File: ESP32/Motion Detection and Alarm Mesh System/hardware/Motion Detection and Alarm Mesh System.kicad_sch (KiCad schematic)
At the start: 0 parts

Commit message: done with block diagram
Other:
- note added: "(MASTER)"
- note added: "(SLAVE 1)"
- note added: "(SLAVE 2)"
- note added: "(SLAVE 3)"
- note added: "BATTERY"
- note added: "BUZZER"
- note added: "CHARGE AND DISCHAGE MODULE"
- note added: "CHARGER"
- note added: "LED INDICATOR"
- note added: "MICROCONTROLLER WITH WIFI COMPATIBILITY"
- note added: "MOTION SENSOR"
- note added: "VOLTAGE REGULATOR"

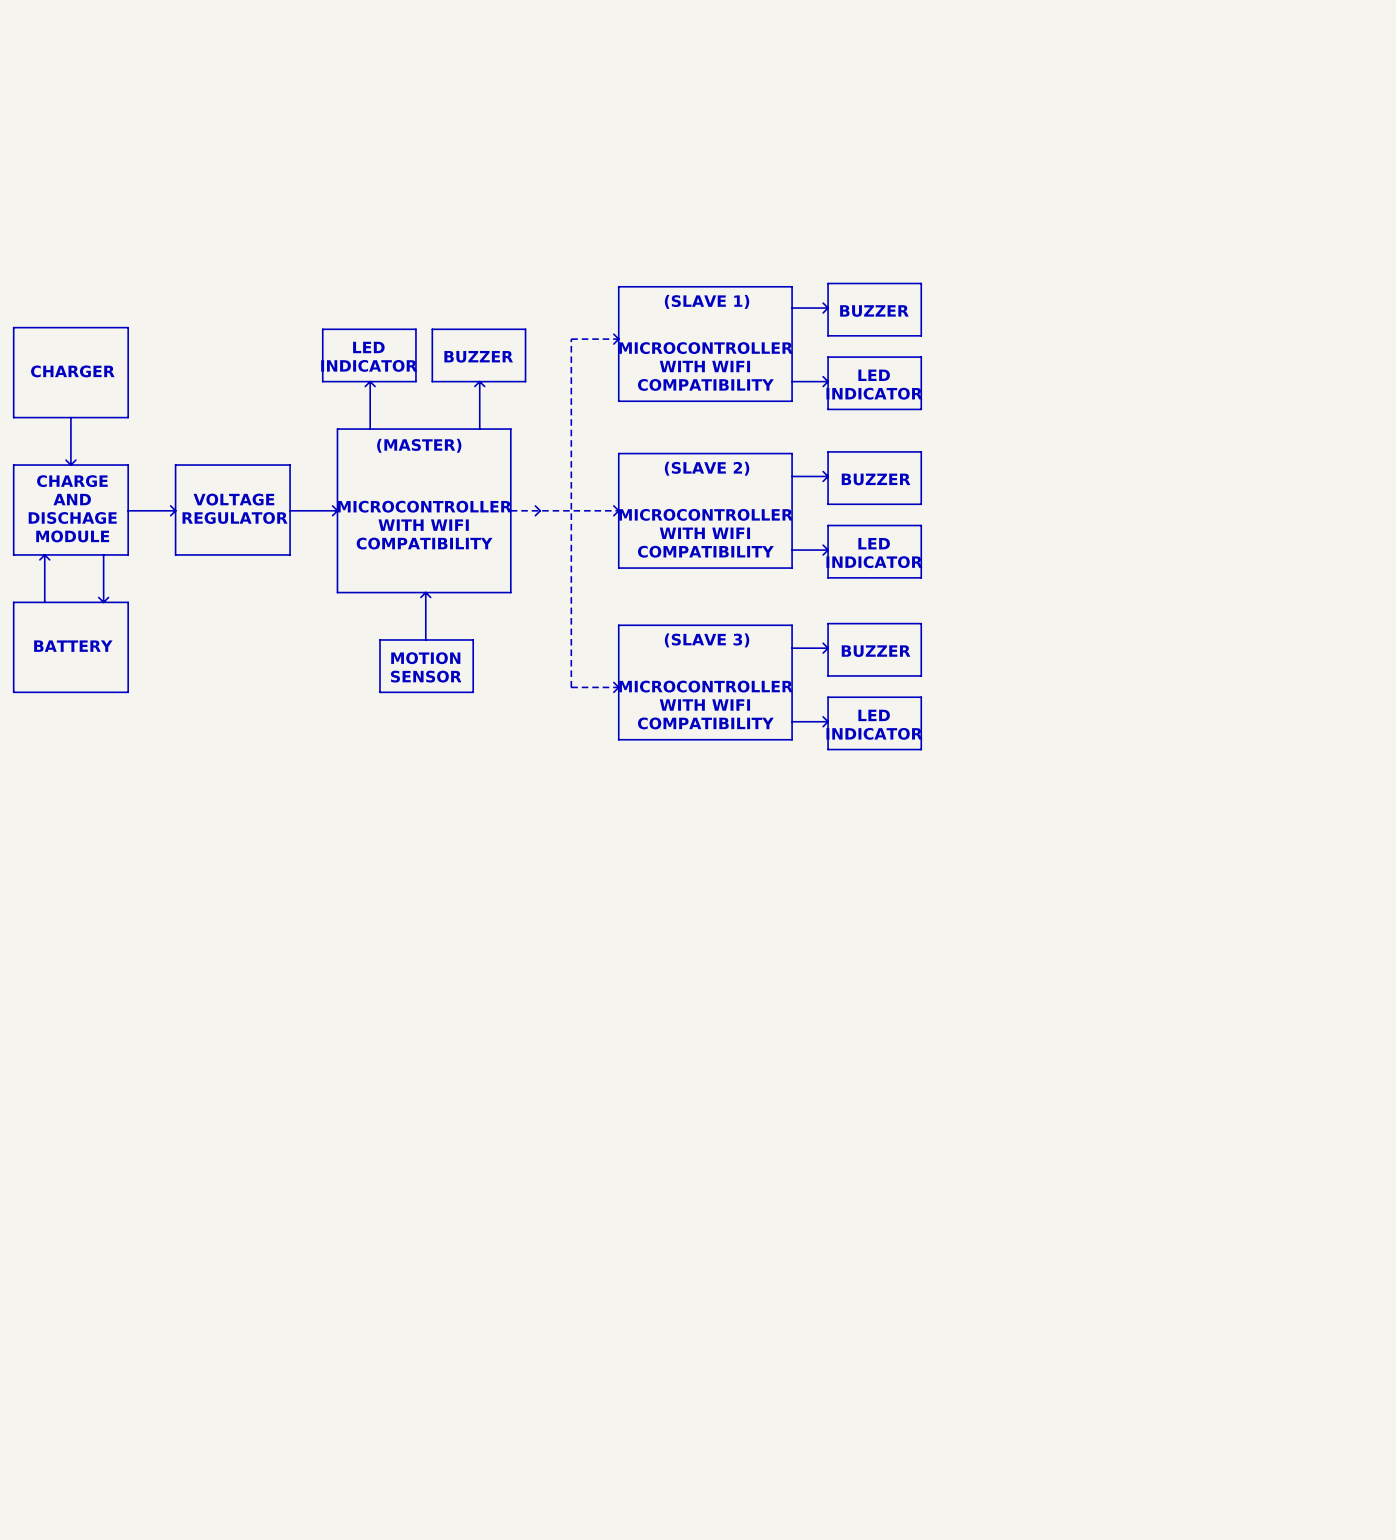
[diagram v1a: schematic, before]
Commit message: Done with Schematic Diagram
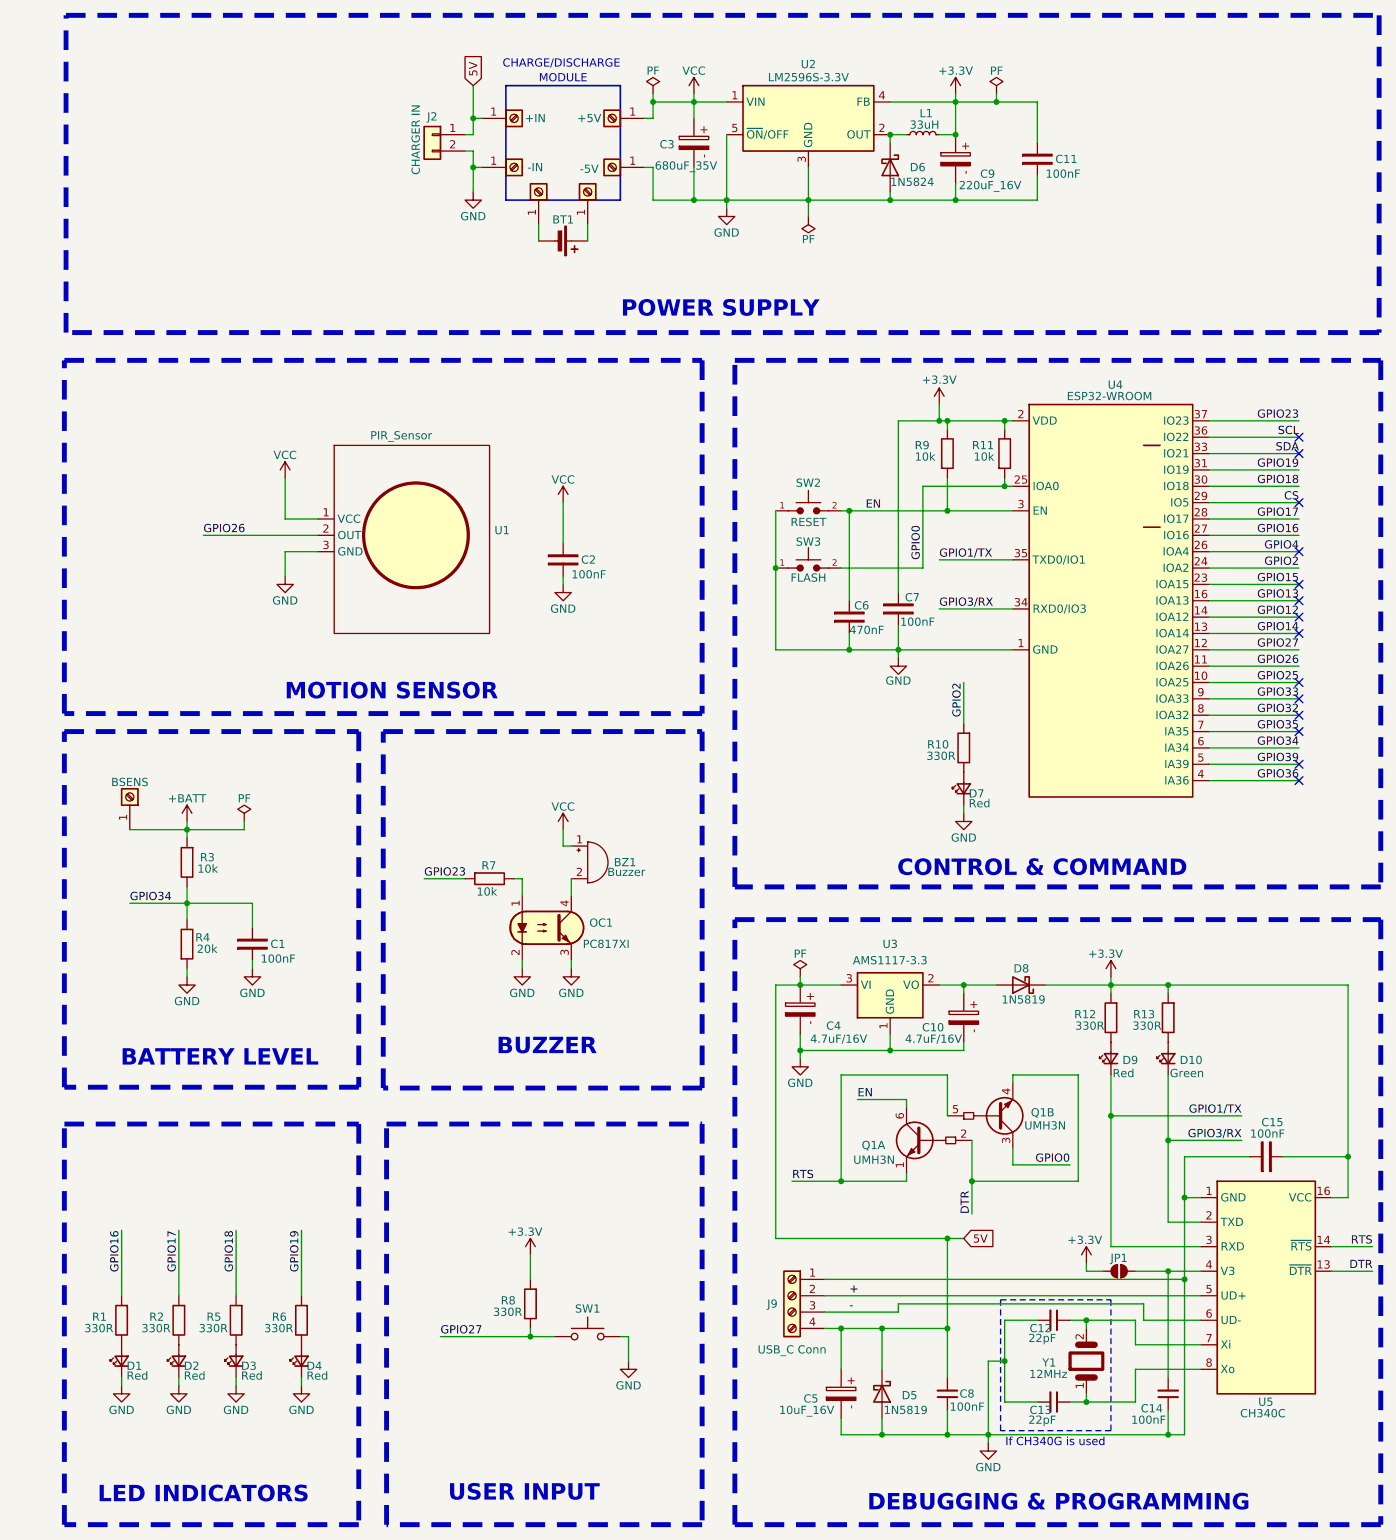
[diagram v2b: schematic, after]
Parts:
- added BT1: Battery_Cell, symbol Device:Battery_Cell
- added BZ1: Buzzer, Buzzer_Beeper:Buzzer_15x7.5RM7.6, symbol Device:Buzzer
- added C1, C11, C15, C2, C7: 100nF, Capacitor_SMD:C_0805_2012Metric_Pad1.18x1.45mm_HandSolder, symbol PCM_SL_Capacitors:104_Ceramic
- added C10, C4: 4.7uF/16V, Capacitor_Tantalum_SMD:CP_EIA-3528-21_Kemet-B_HandSolder, symbol PCM_SL_Capacitors:4.7uF_16V
- added C12, C13: 22pF, Capacitor_SMD:C_0805_2012Metric_Pad1.18x1.45mm_HandSolder, symbol Device:C_Small
- added C14, C8: 100nF, Capacitor_SMD:C_0805_2012Metric_Pad1.18x1.45mm_HandSolder, symbol Device:C_Small
- added C3: 680uF_35V, Capacitor_SMD:CP_Elec_10x12.5, symbol PCM_SL_Capacitors:470uF_35V
- added C5: 10uF_16V, Capacitor_THT:CP_Radial_D5.0mm_P2.00mm, symbol PCM_SL_Capacitors:10uF_16V
- added C6: 470nF, Capacitor_SMD:C_0805_2012Metric_Pad1.18x1.45mm_HandSolder, symbol PCM_SL_Capacitors:104_Ceramic
- added C9: 220uF_16V, Capacitor_SMD:CP_Elec_6.3x7.7, symbol PCM_SL_Capacitors:470uF_35V
- added D1, D2, D3, D4, D7, D9: Red, LED_THT:LED_D3.0mm, symbol SparkFun-LED:LED_Red_0603
- added D10: Green, LED_THT:LED_D3.0mm, symbol SparkFun-LED:LED_Red_0603
- added D5, D8: 1N5819, Diode_SMD:D_SMA, symbol Diode:1N5819
- added D6: 1N5824, Diode_SMD:D_SMA, symbol Diode:1N5822
- added J1: BSENS, Connector_Wire:SolderWire-0.1sqmm_1x01_D0.4mm_OD1mm, symbol Connector:Screw_Terminal_01x01
- added J2: CHARGER IN, symbol Connector_Generic:Conn_01x02
- added J3: +IN, TestPoint:TestPoint_Keystone_5015_Micro_Mini, symbol Connector:Screw_Terminal_01x01
- added J4: -IN, TestPoint:TestPoint_Keystone_5015_Micro_Mini, symbol Connector:Screw_Terminal_01x01
- added J5: -BATT, symbol Connector:Screw_Terminal_01x01
- added J6: +BATT, symbol Connector:Screw_Terminal_01x01
- added J7: +5V, TestPoint:TestPoint_Keystone_5015_Micro_Mini, symbol Connector:Screw_Terminal_01x01
- added J8: -5V, TestPoint:TestPoint_Keystone_5015_Micro_Mini, symbol Connector:Screw_Terminal_01x01
- added J9: USB_C Conn, Connector_PinHeader_2.54mm:PinHeader_1x04_P2.54mm_Vertical, symbol Connector:Screw_Terminal_01x04
- added JP1: ~, Jumper:SolderJumper-2_P1.3mm_Open_Pad1.0x1.5mm, symbol SparkFun-Jumper:SolderJumper_2_Open
- added L1: 33uH, Inductor_SMD:L_12x12mm_H6mm, symbol Device:L_Small
- added OC1: PC817XI, PCM_Package_DIP_AKL:SMDIP-4_W9.53mm, symbol PCM_Optocoupler_AKL:PC817XI
- added Q1: UMH3N, Package_TO_SOT_SMD:SOT-363_SC-70-6, symbol Transistor_BJT:UMH3N
- added R1, R10, R12, R13, R2, R5, R6, R8: 330R, Resistor_SMD:R_0805_2012Metric, symbol PCM_SL_Resistors:1M
- added R11, R3, R7, R9: 10k, Resistor_SMD:R_0805_2012Metric, symbol PCM_SL_Resistors:10k
- added R4: 20k, Resistor_SMD:R_0805_2012Metric, symbol PCM_SL_Resistors:10k
- added SW1: SW_Push, Button_Switch_THT:SW_PUSH_6mm_H13mm, symbol Switch:SW_Push
- added SW2: RESET, Button_Switch_SMD:SW_SPST_CK_KXT3, symbol PCM_SL_Devices:Push_Button
- added SW3: FLASH, Button_Switch_SMD:SW_SPST_CK_KXT3, symbol PCM_SL_Devices:Push_Button
- added U1: PIR_Sensor, PCM_SL_Breakout_Boards:PIR-Sensor, symbol PCM_SL_Breakout_Boards:PIR_Sensor
- added U2: LM2596S-3.3V, Package_TO_SOT_SMD:TO-263-5_TabPin6, symbol Regulator_Switching:LM2596S-3.3
- added U3: AMS1117-3.3, Package_TO_SOT_SMD:SOT-223-3_TabPin2, symbol Regulator_Linear:AMS1117-3.3
- added U4: ESP32-WROOM, RF_Module:ESP32-WROOM-32, symbol SparkFun-RF:ESP32-WROOM
- added U5: CH340C, Package_SO:SOIC-16_3.9x9.9mm_P1.27mm, symbol Interface_USB:CH340C
- added Y1: 12MHz, Crystal:Crystal_HC49-4H_Vertical, symbol PCM_SL_Devices:Crystal_16MHz
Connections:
- new net: C14.2, JP1.1 (A), U5.4 (V3)
- new net: C12.1, U5.7 (Xi), Y1.2
- new net: C13.1, U5.8 (Xo), Y1.1
- new net: OC1.1, R7.2
- new net: D9.2 (A), R12.2
- new net: D3.2 (A), R5.2
- new net: BT1.1 (+), J6.1 (Pin_1)
- new net: C10.1, D8.2 (A), U3.2 (VO)
- new net: D7.2 (A), R10.2
- new net: D2.2 (A), R2.2
- new net: D6.1 (K), L1.1, U2.2 (OUT)
- new net: D1.2 (A), R1.2
- new net: BT1.2 (-), J5.1 (Pin_1)
- new net: BZ1.2 (-), OC1.4
- new net: D4.2 (A), R6.2
- new net: D10.2 (A), R13.2
- new net +: J9.2 (Pin_2), U5.5 (UD+)
- new net +3.3V: C11.2, C15.1, C7.2, C9.1, D8.1 (K), JP1.2 (B), L1.2, R11.2, R12.1, R13.1, R8.1, R9.2, U2.4 (FB), U4.2 (VDD), U5.16 (VCC)
- new net +BATT: J1.1 (Pin_1), R3.1
- new net -: J9.3 (Pin_3), U5.6 (UD-)
- new net 5V: C4.1, C5.1, C8.2, D5.1 (K), J2.1 (Pin_1), J3.1 (Pin_1), J9.4 (Pin_4), U3.3 (VI)
- new net CS: U4.29 (IO5)
- new net DTR: Q1.2 (B1), Q1.4 (E2), U5.13 (~{DTR})
- new net EN: C6.2, Q1.6 (C1), R9.1, SW2.2, U4.3 (EN)
- new net GND: C1.1, C10.2, C11.1, C12.2, C13.2, C14.1, C15.2, C2.1, C3.2, C4.2, C5.2, C6.1, C7.1, C8.1, C9.2, D1.1 (K), D2.1 (K), D3.1 (K), D4.1 (K), D5.2 (A), D6.2 (A), D7.1 (K), J2.2 (Pin_2), J4.1 (Pin_1), J8.1 (Pin_1), J9.1 (Pin_1), OC1.2, OC1.3, R4.1, SW1.2, SW2.1, SW3.1, U1.3 (GND), U2.3 (GND), U2.5 (~{ON}/OFF), U2.6 (GND), U3.1 (GND), U4.1 (GND), U4.15 (GND), U4.38 (GND), U4.39 (GND), U5.1 (GND)
- new net GPIO0: Q1.3 (C2), R11.1, SW3.2, U4.25 (IOA0)
- new net GPIO12: U4.14 (IOA12)
- new net GPIO13: U4.16 (IOA13)
- new net GPIO14: U4.13 (IOA14)
- new net GPIO15: U4.23 (IOA15)
- new net GPIO16: R1.1, U4.27 (IO16)
- new net GPIO17: R2.1, U4.28 (IO17)
- new net GPIO18: R5.1, U4.30 (IO18)
- new net GPIO19: R6.1, U4.31 (IO19)
- new net GPIO1/TX: D9.1 (K), U4.35 (TXD0/IO1), U5.3 (RXD)
- new net GPIO2: R10.1, U4.24 (IOA2)
- new net GPIO23: R7.1, U4.37 (IO23)
- new net GPIO25: U4.10 (IOA25)
- new net GPIO26: U1.2 (OUT), U4.11 (IOA26)
- new net GPIO27: R8.2, SW1.1, U4.12 (IOA27)
- new net GPIO32: U4.8 (IOA32)
- new net GPIO33: U4.9 (IOA33)
- new net GPIO34: C1.2, R3.2, R4.2, U4.6 (IA34)
- new net GPIO35: U4.7 (IA35)
- new net GPIO36: U4.4 (IA36)
- new net GPIO39: U4.5 (IA39)
- new net GPIO3/RX: D10.1 (K), U4.34 (RXD0/IO3), U5.2 (TXD)
- new net GPIO4: U4.26 (IOA4)
- new net RTS: Q1.1 (E1), Q1.5 (B2), U5.14 (~{RTS})
- new net SCL: U4.36 (IO22)
- new net SDA: U4.33 (IO21)
- new net VCC: BZ1.1 (+), C2.2, C3.1, J7.1 (Pin_1), U1.1 (VCC), U2.1 (VIN)
- no-connect marks 0 -> 14
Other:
- note added: "BATTERY LEVEL"
- note added: "CHARGE/DISCHARGE"
- note added: "CONTROL & COMMAND"
- note added: "DEBUGGING & PROGRAMMING"
- note added: "If CH340G is used"
- note added: "LED INDICATORS"
- note added: "MODULE"
- note added: "POWER SUPPLY"
- note added: "USER INPUT"
- note removed: "(MASTER)"
- note removed: "(SLAVE 1)"
- note removed: "(SLAVE 2)"
- note removed: "(SLAVE 3)"
- note removed: "BATTERY"
- note removed: "CHARGE AND DISCHAGE MODULE"
- note removed: "CHARGER"
- note removed: "LED INDICATOR"
- note removed: "MICROCONTROLLER WITH WIFI COMPATIBILITY"
- note removed: "VOLTAGE REGULATOR"
